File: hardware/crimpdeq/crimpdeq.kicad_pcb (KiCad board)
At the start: 2 copper layers, 52 parts, among them J2 USB4105-GF-A, Q1 S8550, Q2 DMG3415U, SW1 SW_Push, SW2 SW_Push, U1 ESP32-C3-MINI-1, U2 MCP73831T-2ACI/OT, U3 HX711, U4 Rust_Board, U6 SY8088, Y1 32.768Hz

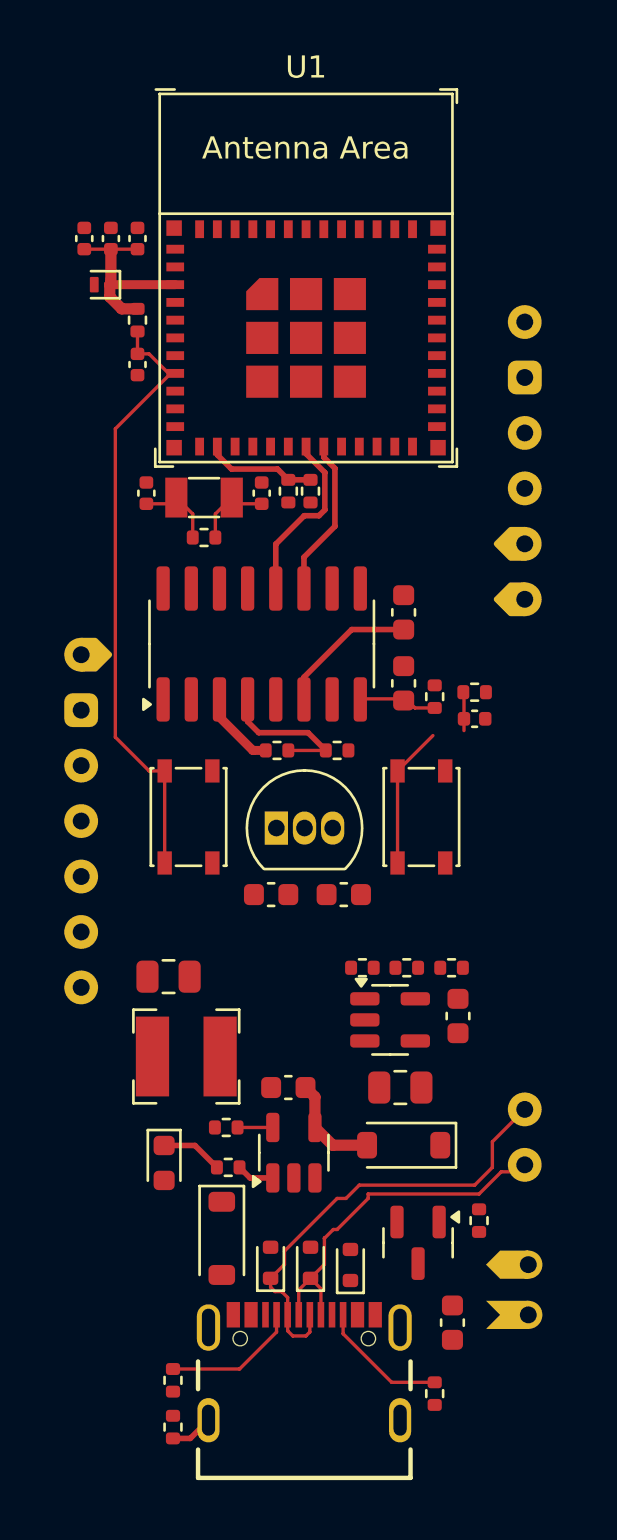
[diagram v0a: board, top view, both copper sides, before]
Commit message: pcb: Update layout
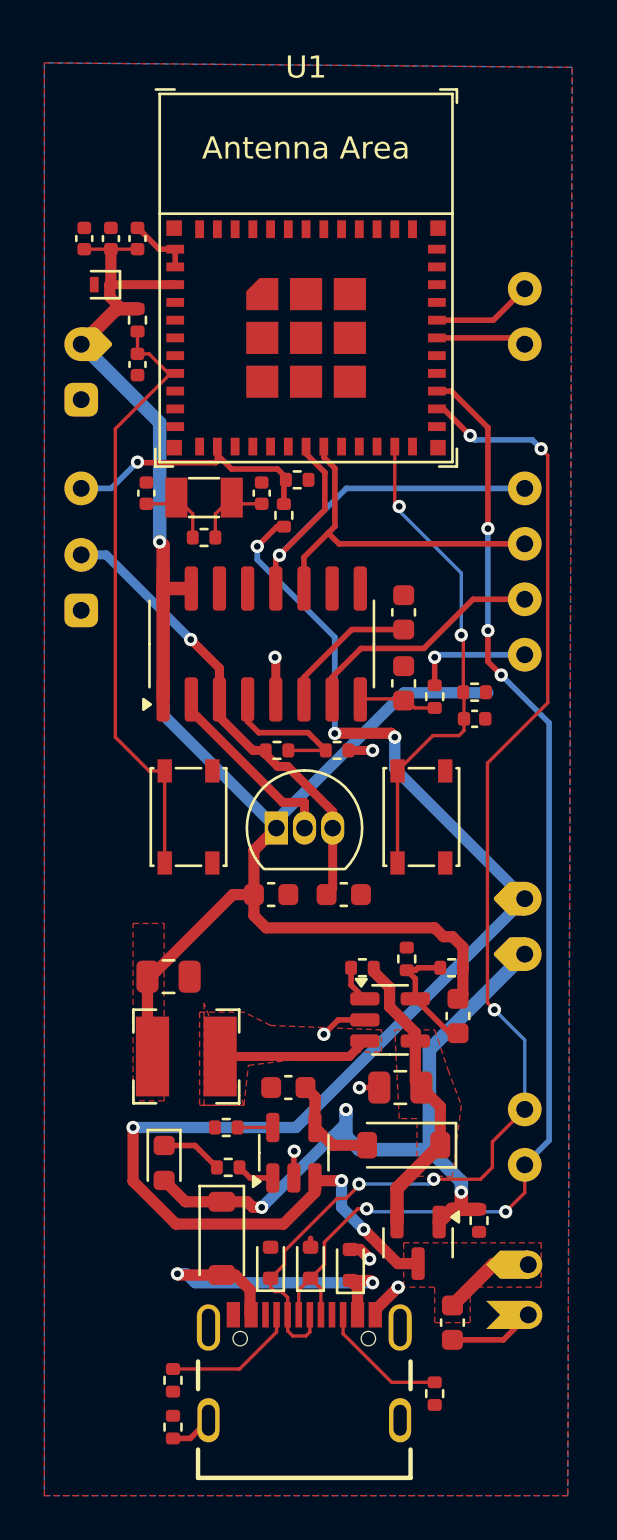
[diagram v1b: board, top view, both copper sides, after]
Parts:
- moved R12 1.62 mm to (139.8, 66.4)
- moved R11 0.65 mm to (140.4, 64.8), turned to 0 degrees
- moved R16 0.40 mm to (145.3, 86.4), turned to 90 degrees
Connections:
- U1 pad 49: GND -> (no net)
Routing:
- net +BATT: track 0.00 -> 69.7 mm, vias 0 -> 6
- net +3V3: track 8.99 -> 77.7 mm, vias 0 -> 1
- net USB_D+: track 16.3 -> 55.2 mm, vias 0 -> 5
- net USB_D-: track 20.5 -> 57.7 mm, vias 0 -> 5
- net VBUS: track 4.48 -> 36.9 mm, vias 0 -> 3
- net E+: track 4.17 -> 22.0 mm, vias 0 -> 1
- net GND: track 1.00 -> 18.2 mm, vias 0 -> 7
- net Net-(D8-A): track 0.00 -> 16.4 mm, vias 0 -> 2
- net IO9_BOOT: track 8.15 -> 22.0 mm, vias 0 -> 2
- net +5V: track 0.00 -> 13.5 mm
- net IO4_DATA: track 8.47 -> 20.4 mm, vias 0 -> 1
- net A-: track 0.00 -> 11.1 mm
- net IO5_SCK: track 7.19 -> 16.2 mm
- net Net-(Q1-B): track 0.00 -> 8.49 mm
- net IO1_ADC: track 5.04 -> 12.4 mm, vias 0 -> 1
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- added copper zone on F.Cu, net +3V3
- added copper zone on F.Cu, net +5V
- added copper zone on F.Cu, net +BATT
- added copper zone on F.Cu, net /Buck_Coil
- added copper zone on B.Cu, net GND
- added copper zone on F.Cu, net GND
